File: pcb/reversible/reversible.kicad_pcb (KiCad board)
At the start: 2 copper layers, 31 parts, among them J2 5PIN, U1 ProMicro

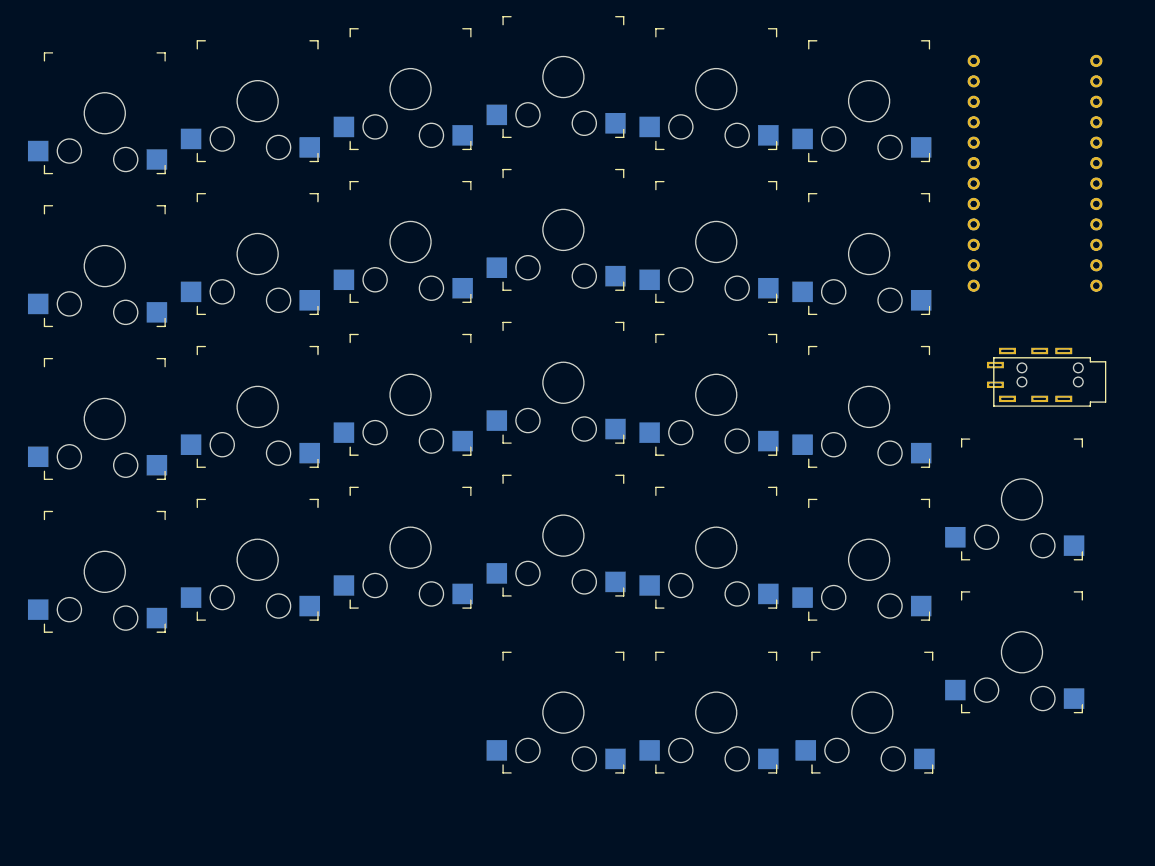
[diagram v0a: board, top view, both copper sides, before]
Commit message: layout designed
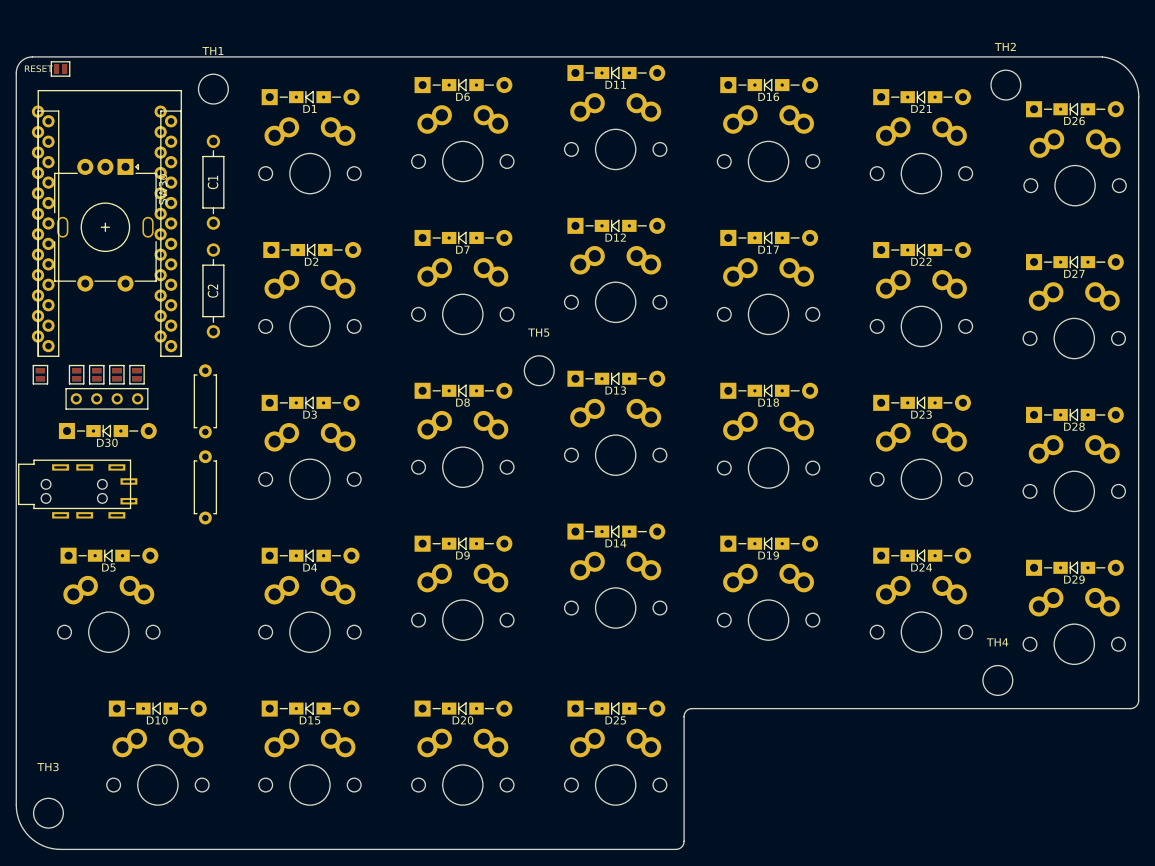
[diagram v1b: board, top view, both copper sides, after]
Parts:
- removed J2: 5PIN, lowProfile:TRRS_JACK_MJ4PP9
- removed REF** (x29): Gateron_Low_Profile_Socket, lowProfileSplit:Gateron_Low_Profile_Socket
- added C1: 100nF, lowProfile:RESISTOR, F.Cu at (79.5, 60.6)
- added C2: 100nF, lowProfile:RESISTOR, F.Cu at (79.5, 74.1)
- added D1: 1N4148/1N4148W, lowProfile:Diode_TH_SOD123, F.Cu at (91.5, 50.0)
- added D10: 1N4148/1N4148W, lowProfile:Diode_TH_SOD123, F.Cu at (72.5, 126.0)
- added D11: 1N4148/1N4148W, lowProfile:Diode_TH_SOD123, F.Cu at (129.5, 47.0)
- added D12: 1N4148/1N4148W, lowProfile:Diode_TH_SOD123, F.Cu at (129.5, 66.0)
- added D13: 1N4148/1N4148W, lowProfile:Diode_TH_SOD123, F.Cu at (129.5, 85.0)
- added D14: 1N4148/1N4148W, lowProfile:Diode_TH_SOD123, F.Cu at (129.5, 104.0)
- added D15: 1N4148/1N4148W, lowProfile:Diode_TH_SOD123, F.Cu at (91.5, 126.0)
- added D16: 1N4148/1N4148W, lowProfile:Diode_TH_SOD123, F.Cu at (148.5, 48.5)
- added D17: 1N4148/1N4148W, lowProfile:Diode_TH_SOD123, F.Cu at (148.5, 67.5)
- added D18: 1N4148/1N4148W, lowProfile:Diode_TH_SOD123, F.Cu at (148.5, 86.5)
- added D19: 1N4148/1N4148W, lowProfile:Diode_TH_SOD123, F.Cu at (148.5, 105.5)
- added D2: 1N4148/1N4148W, lowProfile:Diode_TH_SOD123, F.Cu at (91.7, 69.0)
- added D20: 1N4148/1N4148W, lowProfile:Diode_TH_SOD123, F.Cu at (110.5, 126.0)
- added D21: 1N4148/1N4148W, lowProfile:Diode_TH_SOD123, F.Cu at (167.5, 50.0)
- added D22: 1N4148/1N4148W, lowProfile:Diode_TH_SOD123, F.Cu at (167.5, 69.0)
- added D23: 1N4148/1N4148W, lowProfile:Diode_TH_SOD123, F.Cu at (167.5, 88.0)
- added D24: 1N4148/1N4148W, lowProfile:Diode_TH_SOD123, F.Cu at (167.5, 107.0)
- added D25: 1N4148/1N4148W, lowProfile:Diode_TH_SOD123, F.Cu at (129.5, 126.0)
- added D26: 1N4148/1N4148W, lowProfile:Diode_TH_SOD123, F.Cu at (186.5, 51.5)
- added D27: 1N4148/1N4148W, lowProfile:Diode_TH_SOD123, F.Cu at (186.5, 70.5)
- added D28: 1N4148/1N4148W, lowProfile:Diode_TH_SOD123, F.Cu at (186.5, 89.5)
- added D29: 1N4148/1N4148W, lowProfile:Diode_TH_SOD123, F.Cu at (186.5, 108.5)
- added D3: 1N4148/1N4148W, lowProfile:Diode_TH_SOD123, F.Cu at (91.5, 88.0)
- added D30: 1N4148/1N4148W, lowProfile:Diode_TH_SOD123, F.Cu at (66.3, 91.5)
- added D4: 1N4148/1N4148W, lowProfile:Diode_TH_SOD123, F.Cu at (91.5, 107.0)
- added D5: 1N4148/1N4148W, lowProfile:Diode_TH_SOD123, F.Cu at (66.5, 107.0)
- added D6: 1N4148/1N4148W, lowProfile:Diode_TH_SOD123, F.Cu at (110.5, 48.5)
- added D7: 1N4148/1N4148W, lowProfile:Diode_TH_SOD123, F.Cu at (110.5, 67.5)
- added D8: 1N4148/1N4148W, lowProfile:Diode_TH_SOD123, F.Cu at (110.5, 86.5)
- added D9: 1N4148/1N4148W, lowProfile:Diode_TH_SOD123, F.Cu at (110.5, 105.5)
- added J1: PJ-320A, lowProfile:TRRS_JACK_MJ4PP9, F.Cu at (57.2, 98.1)
- added JP1: RESET, lowProfile:Jumper, B.Cu at (60.5, 46.5)
- added JP10: Jumper_NO_Small, lowProfile:Jumper, B.Cu at (70.0, 84.5)
- added JP11: LEFT, lowProfile:Jumper, F.Cu at (58.0, 84.5)
- added JP12: RIGHT, lowProfile:Jumper, B.Cu at (58.0, 84.5)
- added JP2: RESET, lowProfile:Jumper, F.Cu at (60.5, 46.5)
- added JP3: Jumper_NO_Small, lowProfile:Jumper, F.Cu at (62.5, 84.5)
- added JP4: Jumper_NO_Small, lowProfile:Jumper, F.Cu at (65.0, 84.5)
- added JP5: Jumper_NO_Small, lowProfile:Jumper, F.Cu at (67.5, 84.5)
- added JP6: Jumper_NO_Small, lowProfile:Jumper, F.Cu at (70.0, 84.5)
- added JP7: Jumper_NO_Small, lowProfile:Jumper, B.Cu at (62.5, 84.5)
- added JP8: Jumper_NO_Small, lowProfile:Jumper, B.Cu at (65.0, 84.5)
- added JP9: Jumper_NO_Small, lowProfile:Jumper, B.Cu at (67.5, 84.5)
- added P1: OLED, lowProfile:OLED_4Pin, F.Cu at (62.5, 87.5)
- added R1: 4k7, Resistor_THT:R_Axial_DIN0207_L6.3mm_D2.5mm_P7.62mm_Horizontal, F.Cu at (78.5, 91.6)
- added R2: 4k7, Resistor_THT:R_Axial_DIN0207_L6.3mm_D2.5mm_P7.62mm_Horizontal, F.Cu at (78.5, 102.3)
- added SW1: Kailh hotswap MX socket, lowProfile:Gateron_Low_Profile_Socket, F.Cu at (91.5, 59.5)
- added SW10: Kailh hotswap MX socket, lowProfile:Gateron_Low_Profile_Socket, F.Cu at (72.6, 135.5)
- added SW11: Kailh hotswap MX socket, lowProfile:Gateron_Low_Profile_Socket, F.Cu at (129.5, 56.5)
- added SW12: Kailh hotswap MX socket, lowProfile:Gateron_Low_Profile_Socket, F.Cu at (129.5, 75.5)
- added SW13: Kailh hotswap MX socket, lowProfile:Gateron_Low_Profile_Socket, F.Cu at (129.5, 94.5)
- added SW14: Kailh hotswap MX socket, lowProfile:Gateron_Low_Profile_Socket, F.Cu at (129.5, 113.5)
- added SW15: Kailh hotswap MX socket, lowProfile:Gateron_Low_Profile_Socket, F.Cu at (91.5, 135.5)
- added SW16: Kailh hotswap MX socket, lowProfile:Gateron_Low_Profile_Socket, F.Cu at (148.5, 58.0)
- added SW17: Kailh hotswap MX socket, lowProfile:Gateron_Low_Profile_Socket, F.Cu at (148.5, 77.0)
- added SW18: Kailh hotswap MX socket, lowProfile:Gateron_Low_Profile_Socket, F.Cu at (148.5, 96.1)
- added SW19: Kailh hotswap MX socket, lowProfile:Gateron_Low_Profile_Socket, F.Cu at (148.5, 115.0)
- added SW2: Kailh hotswap MX socket, lowProfile:Gateron_Low_Profile_Socket, F.Cu at (91.5, 78.5)
- added SW20: Kailh hotswap MX socket, lowProfile:Gateron_Low_Profile_Socket, F.Cu at (110.5, 135.5)
- added SW21: Kailh hotswap MX socket, lowProfile:Gateron_Low_Profile_Socket, F.Cu at (167.5, 59.5)
- added SW22: Kailh hotswap MX socket, lowProfile:Gateron_Low_Profile_Socket, F.Cu at (167.5, 78.5)
- added SW23: Kailh hotswap MX socket, lowProfile:Gateron_Low_Profile_Socket, F.Cu at (167.5, 97.5)
- added SW24: Kailh hotswap MX socket, lowProfile:Gateron_Low_Profile_Socket, F.Cu at (167.5, 116.5)
- added SW25: Kailh hotswap MX socket, lowProfile:Gateron_Low_Profile_Socket, F.Cu at (129.5, 135.5)
- added SW26: Kailh hotswap MX socket, lowProfile:Gateron_Low_Profile_Socket, F.Cu at (186.6, 61.0)
- added SW27: Kailh hotswap MX socket, lowProfile:Gateron_Low_Profile_Socket, F.Cu at (186.5, 80.0)
- added SW28: Kailh hotswap MX socket, lowProfile:Gateron_Low_Profile_Socket, F.Cu at (186.5, 99.0)
- added SW29: Kailh hotswap MX socket, lowProfile:Gateron_Low_Profile_Socket, F.Cu at (186.5, 118.0)
- added SW3: Kailh hotswap MX socket, lowProfile:Gateron_Low_Profile_Socket, F.Cu at (91.5, 97.5)
- added SW30: Rotary_Encoder_Switch, lowProfile:RotaryEncoder_Alps_EC12E-Switch_Vertical_H20mm, F.Cu at (66.1, 66.2)
- added SW4: Kailh hotswap MX socket, lowProfile:Gateron_Low_Profile_Socket, F.Cu at (91.5, 116.5)
- added SW5: Kailh hotswap MX socket, lowProfile:Gateron_Low_Profile_Socket, F.Cu at (66.5, 116.5)
- added SW6: Kailh hotswap MX socket, lowProfile:Gateron_Low_Profile_Socket, F.Cu at (110.5, 58.0)
- added SW7: Kailh hotswap MX socket, lowProfile:Gateron_Low_Profile_Socket, F.Cu at (110.5, 77.0)
- added SW8: Kailh hotswap MX socket, lowProfile:Gateron_Low_Profile_Socket, F.Cu at (110.5, 96.0)
- added SW9: Kailh hotswap MX socket, lowProfile:Gateron_Low_Profile_Socket, F.Cu at (110.5, 115.0)
- added TH1: HOLE, MountingHole:MountingHole_3.7mm, F.Cu at (79.5, 49.0)
- added TH2: HOLE, MountingHole:MountingHole_3.7mm, F.Cu at (178.0, 48.5)
- added TH3: HOLE, MountingHole:MountingHole_3.7mm, F.Cu at (59.0, 139.0)
- added TH4: HOLE, MountingHole:MountingHole_3.7mm, F.Cu at (177.0, 122.5)
- added TH5: HOLE, MountingHole:MountingHole_3.7mm, F.Cu at (120.0, 84.0)
- U1: footprint lowProfile:ProMicro_rev -> lowProfile:ProMicro_rev2
- moved U1 115.3 mm to (66.5, 66.6)
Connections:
- U1 pad 1: (no net) -> unconnected-(U1-TX0/PD3-Pad1)
- U1 pad 10: (no net) -> row3
- U1 pad 11: (no net) -> row4
- U1 pad 12: (no net) -> Hand
- U1 pad 13: (no net) -> col3
- U1 pad 14: (no net) -> col1
- U1 pad 15: (no net) -> col2
- U1 pad 16: (no net) -> col0
- U1 pad 17: (no net) -> col4
- U1 pad 18: (no net) -> col5
- U1 pad 19: (no net) -> A
- U1 pad 2: (no net) -> DATA
- U1 pad 20: (no net) -> B
- U1 pad 21: (no net) -> VCC
- U1 pad 22: (no net) -> RESET
- U1 pad 23: (no net) -> GND
- U1 pad 24: (no net) -> unconnected-(U1-RAW-Pad24)
- U1 pad 3: (no net) -> GND
- U1 pad 4: (no net) -> GND
- U1 pad 5: (no net) -> SDA
- U1 pad 6: (no net) -> SCL
- U1 pad 7: (no net) -> row0
- U1 pad 8: (no net) -> row1
- U1 pad 9: (no net) -> row2
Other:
- board outline added: 139.5 x 98.5 mm
